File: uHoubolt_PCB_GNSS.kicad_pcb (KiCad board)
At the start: 2 copper layers, 90 x 90 mm, 5 parts, among them J1 UART, U1 SAM-M8Q

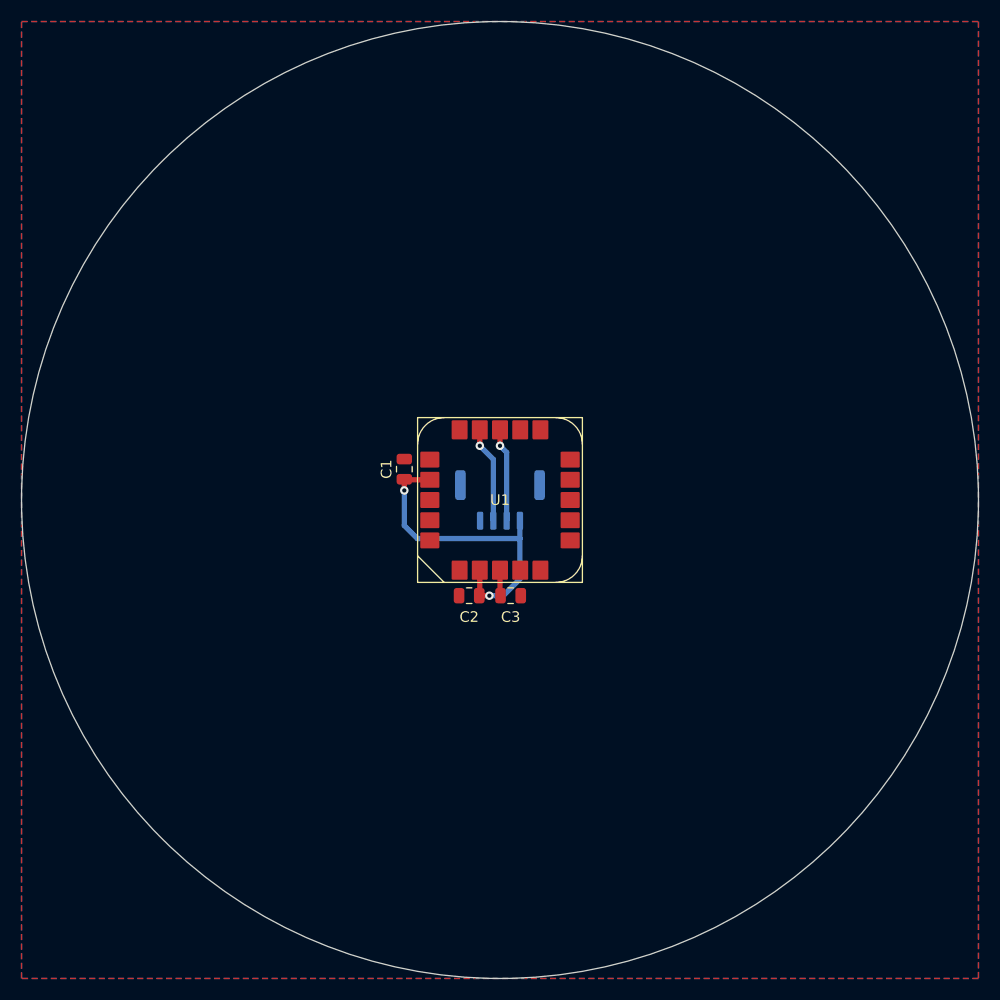
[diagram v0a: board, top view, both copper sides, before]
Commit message: first revision done
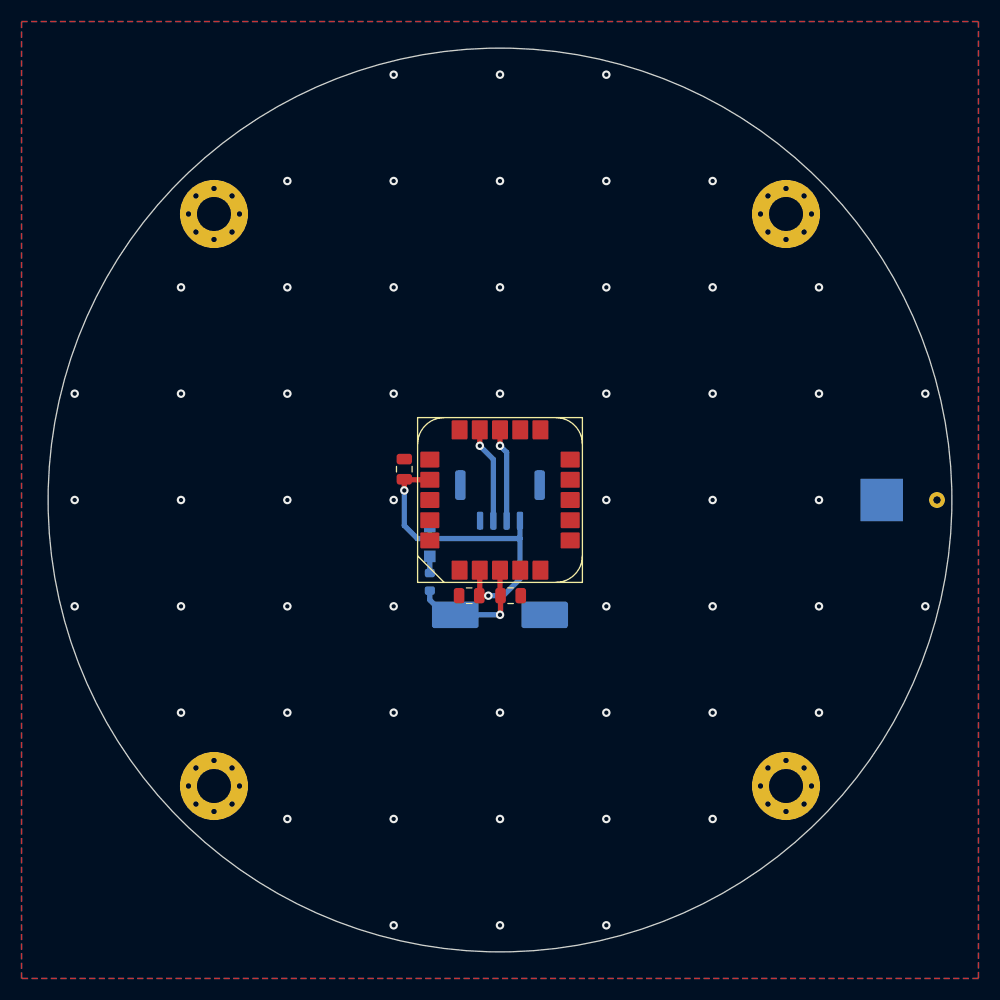
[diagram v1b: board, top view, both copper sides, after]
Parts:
- added C4: 470m, Capacitor_SMD:CP_Elec_10x10.5, B.Cu at (150.0, 110.8)
- added D1: Schottky, Diode_SMD:D_SOD-123F, B.Cu at (143.4, 103.9)
- added H1: M3, MountingHole:MountingHole_3.2mm_M3_Pad_Via, F.Cu at (176.9, 73.1)
- added H2: M3, MountingHole:MountingHole_3.2mm_M3_Pad_Via, F.Cu at (123.1, 73.1)
- added H3: M3, MountingHole:MountingHole_3.2mm_M3_Pad_Via, F.Cu at (123.1, 126.9)
- added H4: M3, MountingHole:MountingHole_3.2mm_M3_Pad_Via, F.Cu at (176.9, 126.9)
- added J2: GND, TestPoint:TestPoint_Pad_4.0x4.0mm, B.Cu at (185.9, 100.0)
- added J3: ANT, TestPoint:TestPoint_THTPad_D1.5mm_Drill0.7mm, B.Cu at (191.1, 100.0)
- added R1: 330, Resistor_SMD:R_0603_1608Metric, B.Cu at (143.4, 107.7)
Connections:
- C3 pad 1: +3V3 -> Net-(C3-Pad1)
- U1 pad 3: +3V3 -> Net-(C3-Pad1)
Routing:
- net Net-(C3-Pad1): track 0.00 -> 12.3 mm, vias 0 -> 1
- net Net-(D1-Pad1): track 0.00 -> 1.58 mm
- net +3V3: track 32.9 -> 31.7 mm
- net GND: vias 0 -> 54
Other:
- board size 90 x 90 mm -> 85 x 85 mm
- board text added: "GND RxD TxD 3V3"
